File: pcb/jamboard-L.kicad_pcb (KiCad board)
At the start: 2 copper layers, 141.5 x 117.8 mm, 118 parts, among them J1 OLED_128x32, J2 RJ45, U1 Pico

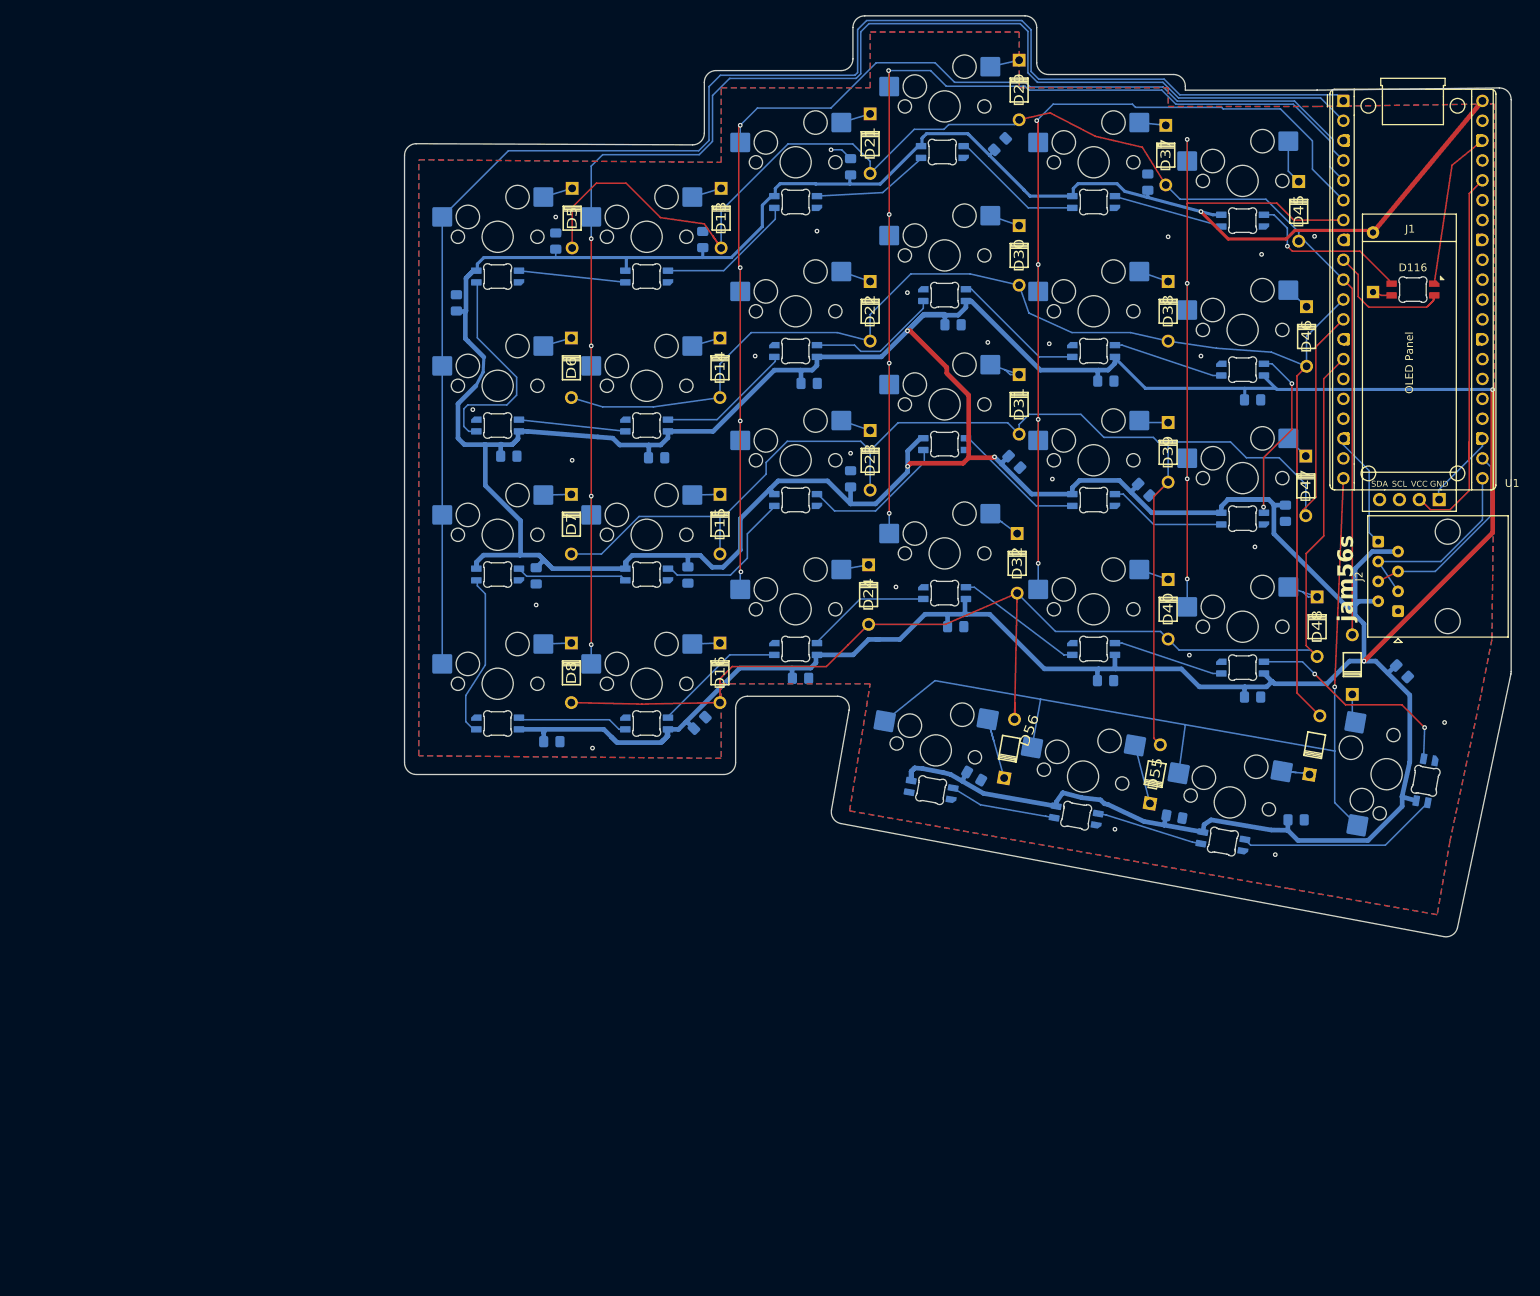
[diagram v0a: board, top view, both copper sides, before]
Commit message: rust firmware attempt1
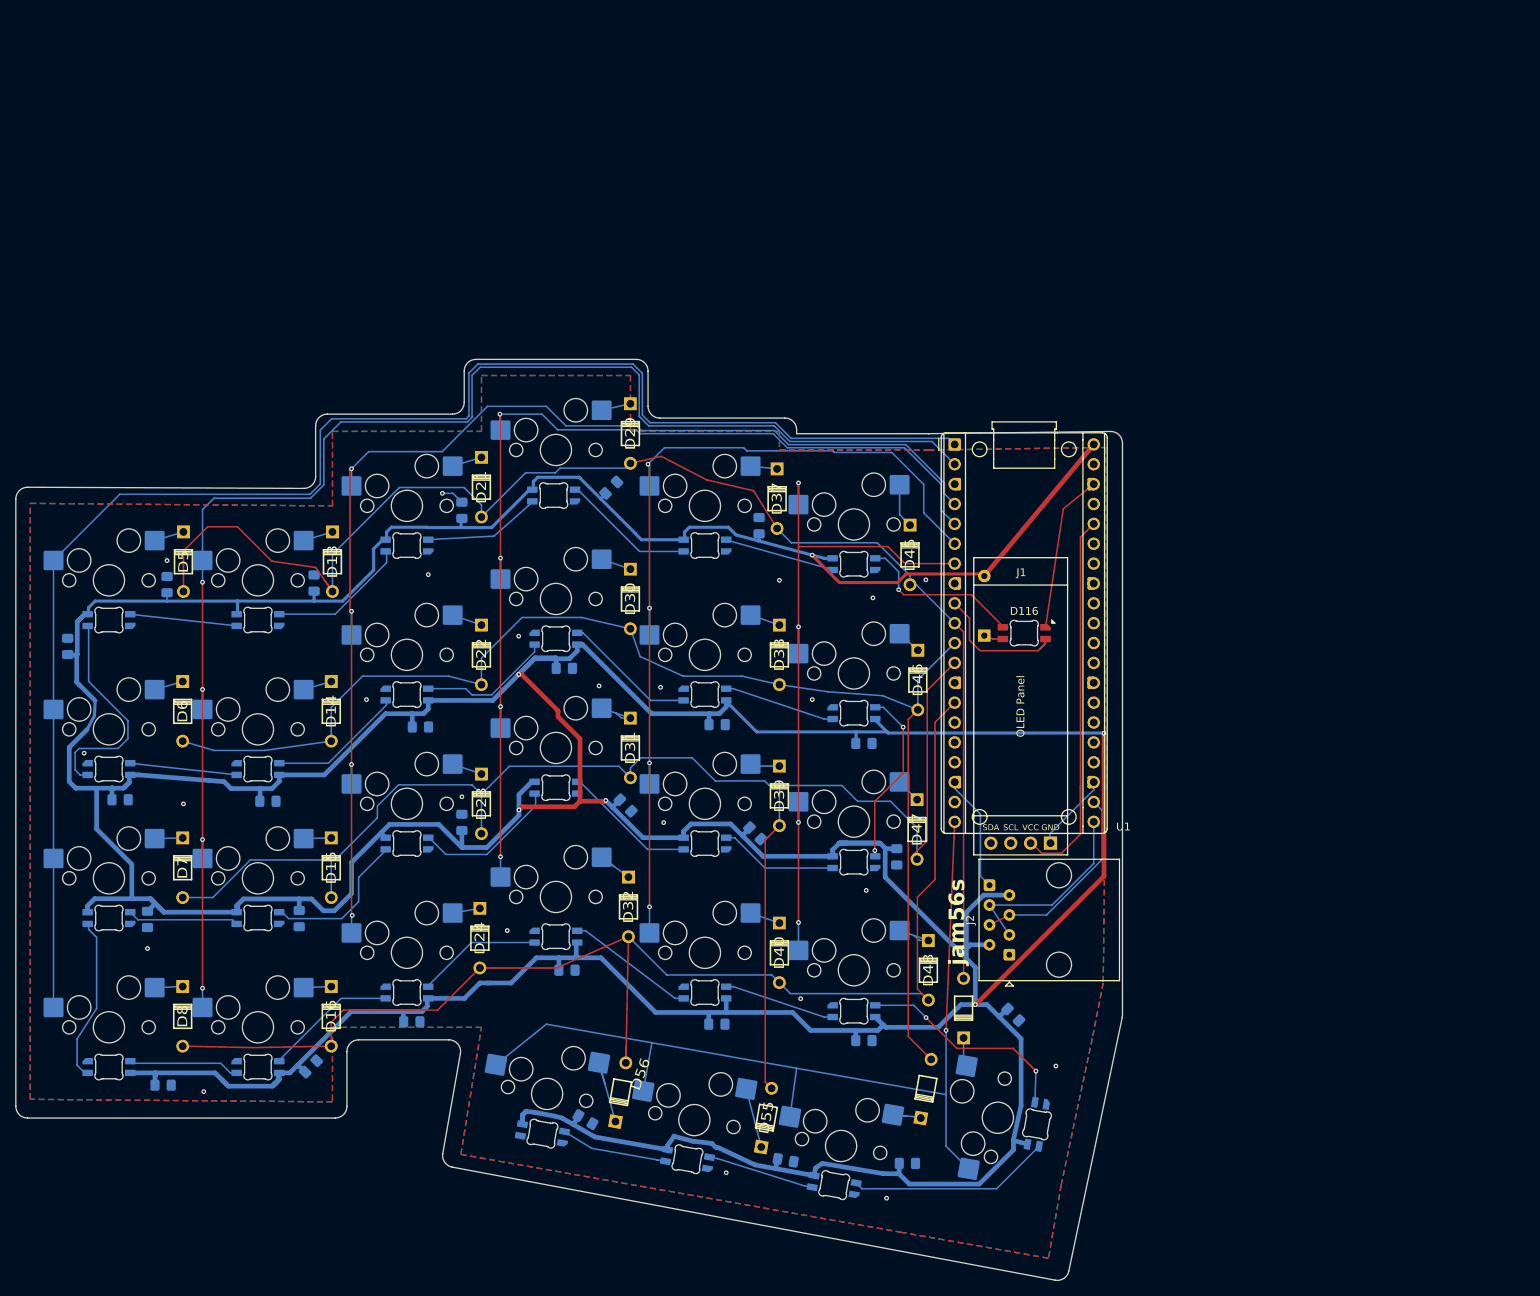
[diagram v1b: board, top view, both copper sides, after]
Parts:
- moved C1 66.3 mm to (-85.5, 45.7)
- moved C10 66.3 mm to (-110.4, 63.9)
- moved C13 66.3 mm to (-67.9, 88.0)
- moved C14 66.3 mm to (-86.0, 85.0)
- moved C16 66.3 mm to (-123.5, 83.6)
- moved C17 66.3 mm to (-144.3, 95.9)
- moved C20 66.3 mm to (-142.8, 114.8)
- moved C21 66.3 mm to (-129.9, 109.1)
- moved C22 66.3 mm to (-110.1, 102.5)
- moved C23 66.3 mm to (-90.9, 109.4)
- moved C3 66.3 mm to (-123.5, 43.7)
- moved C6 66.3 mm to (-173.9, 61.1)
- moved C8 66.3 mm to (-148.3, 80.9)
- moved C9 66.3 mm to (-128.8, 71.4)
- moved D100 66.3 mm to (-94.7, 126.7)
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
